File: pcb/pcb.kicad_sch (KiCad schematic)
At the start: 22 parts, among them J1 USB4085-GF-A_REVB, J2 AudioJack4, J3 AudioJack4, J4 Conn_01x03_Socket, SW1 SW_Push, SW2 SW_Push, SW3 SW_Push, SW4 SW_Push, SW5 SW_Push, SW6 SW_Push, SW7 RotaryEncoder_Switch, SW8 RotaryEncoder_Switch, U1 Pico, U2 Pico, U3 LM1117MP-5.0

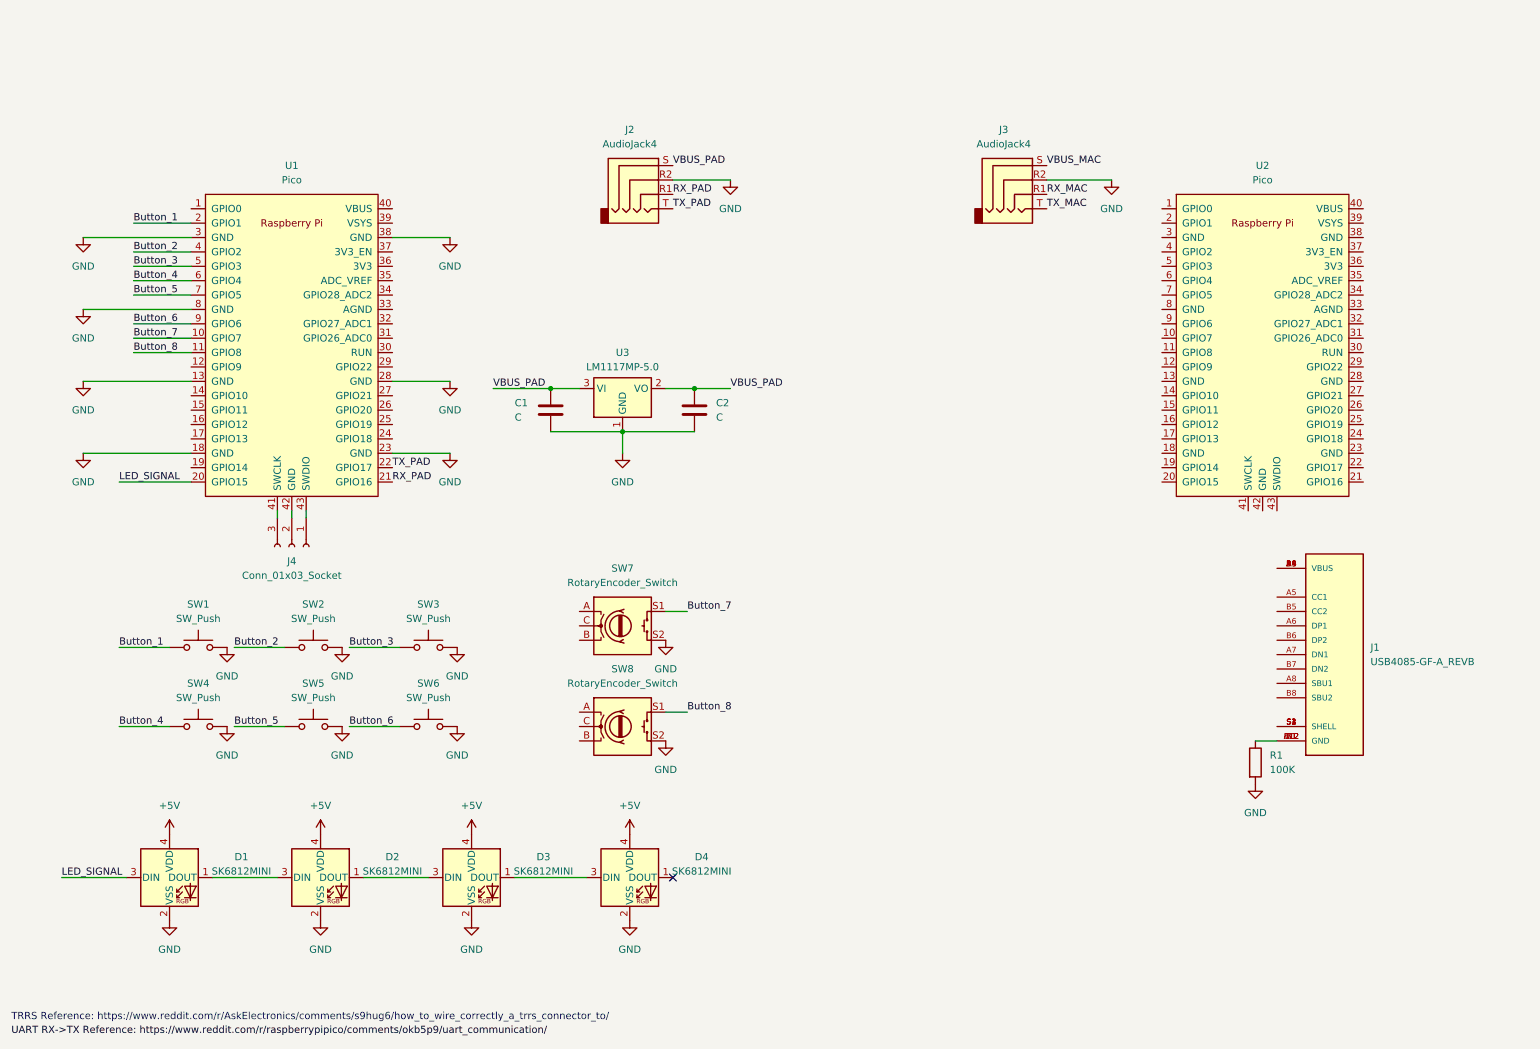
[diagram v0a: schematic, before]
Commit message: Changes on MACmini
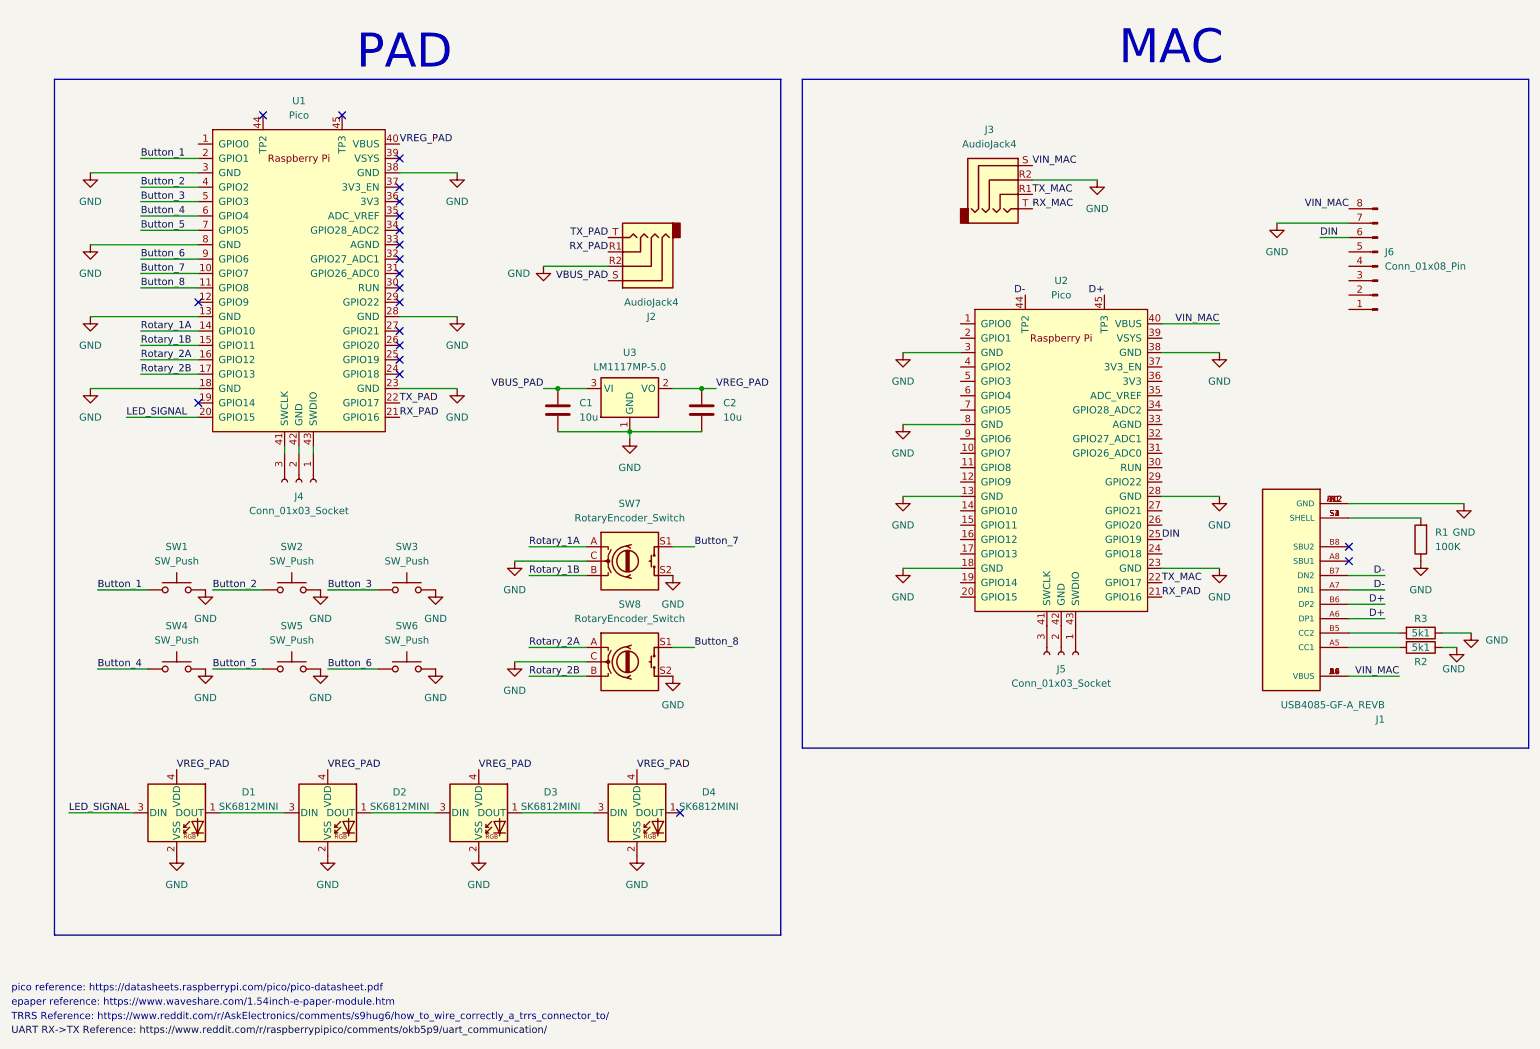
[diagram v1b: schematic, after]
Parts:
- added J5: Conn_01x03_Socket, symbol Connector:Conn_01x03_Socket
- added J6: Conn_01x08_Pin, symbol Connector:Conn_01x08_Pin
- added R2, R3: 5k1, Capacitor_SMD:C_0603_1608Metric, symbol Device:R
- C1, C2: value C -> 10u; footprint (none) -> Capacitor_SMD:C_0603_1608Metric
- D1, D2, D3, D4: footprint LED_SMD:LED_SK6812MINI_PLCC4_3.5x3.5mm_P1.75mm -> LED_SMD:LED_WS2812B_PLCC4_5.0x5.0mm_P3.2mm
- J2, J3: footprint (none) -> Connector_Audio:Jack_3.5mm_PJ320D_Horizontal
- SW1, SW2, SW3, SW4, SW5, SW6: footprint (none) -> Button_Switch_Keyboard:SW_Cherry_MX_1.00u_PCB
- SW8: footprint (none) -> Rotary_Encoder:RotaryEncoder_Alps_EC11E_Vertical_H20mm
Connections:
- net +5V is gone; now on net VREG_PAD: D1.4 (VDD), D2.4 (VDD), D3.4 (VDD), D4.4 (VDD)
- net VBUS_MAC is gone; now on net VIN_MAC: J3.S
- net GND: now also J1.A1 (GND), J1.A12 (GND), J1.B1 (GND), J1.B12 (GND), R1.1, SW7.C, SW8.C, U2.13 (GND), U2.18 (GND), U2.23 (GND), U2.28 (GND), U2.3 (GND), U2.38 (GND), U2.8 (GND), J6.7 (Pin_7), R2.1, R3.1; no longer R1.2
- net RX_MAC: now also J3.T; no longer J3.R1
- net RX_PAD: now also U2.21 (GPIO16)
- net TX_MAC: now also J3.R1, U2.22 (GPIO17); no longer J3.T
- net VBUS_PAD: no longer C2.1, U3.2 (VO)
- net VIN_MAC: now reaches J1.A4 (VBUS), J1.A9 (VBUS), J1.B4 (VBUS), J1.B9 (VBUS)
- net VIN_MAC: now also U2.40 (VBUS), J6.8 (Pin_8)
- net at J1.A5 (CC1): now also R2.2
- net D+: now reaches J1.A6 (DP1)
- net D+: now also J1.B6 (DP2), U2.45 (TP3)
- net D-: now reaches J1.A7 (DN1)
- net D-: now also J1.B7 (DN2), U2.44 (TP2)
- net at J1.B5 (CC2): now also R3.2
- net at J1.S1 (SHELL), J1.S2 (SHELL), J1.S3 (SHELL)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: now also R1.2
- net Rotary_2A: now reaches SW8.A
- net Rotary_2A: now also U1.16 (GPIO12)
- net Rotary_2B: now reaches SW8.B
- net Rotary_2B: now also U1.17 (GPIO13)
- net DIN: now reaches U2.25 (GPIO19)
- net DIN: now also J6.6 (Pin_6)
- net at U2.41 (SWCLK): now also J5.3 (Pin_3)
- net at U2.42 (GND): now also J5.2 (Pin_2)
- net at U2.43 (SWDIO): now also J5.1 (Pin_1)
- net Rotary_1A: now reaches SW7.A
- net Rotary_1A: now also U1.14 (GPIO10)
- net Rotary_1B: now reaches SW7.B
- net Rotary_1B: now also U1.15 (GPIO11)
- net VREG_PAD: now reaches U1.40 (VBUS)
- net VREG_PAD: now also C2.1, U3.2 (VO)
- no-connect marks 1 -> 21
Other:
- note added: "MAC"
- note added: "PAD"
- note added: "epaper reference: https://www.waveshare.com/1.54inch-e-paper-module.htm"
- note added: "pico reference: https://datasheets.raspberrypi.com/pico/pico-datasheet.pdf"
- moved on the sheet: D1, D2, D3, D4, J1, J2, J3, J4, SW1, SW2, SW3, SW4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
